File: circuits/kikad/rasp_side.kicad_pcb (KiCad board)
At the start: 2 copper layers, 99.7 x 99.7 mm, 84 parts, among them J1 RJ45, J10 RJ45, J2 RJ45, J3 RJ45, J4 RJ45, J5 RJ45, J6 RJ45, J7 RJ45, J8 RJ45, J9 RJ45

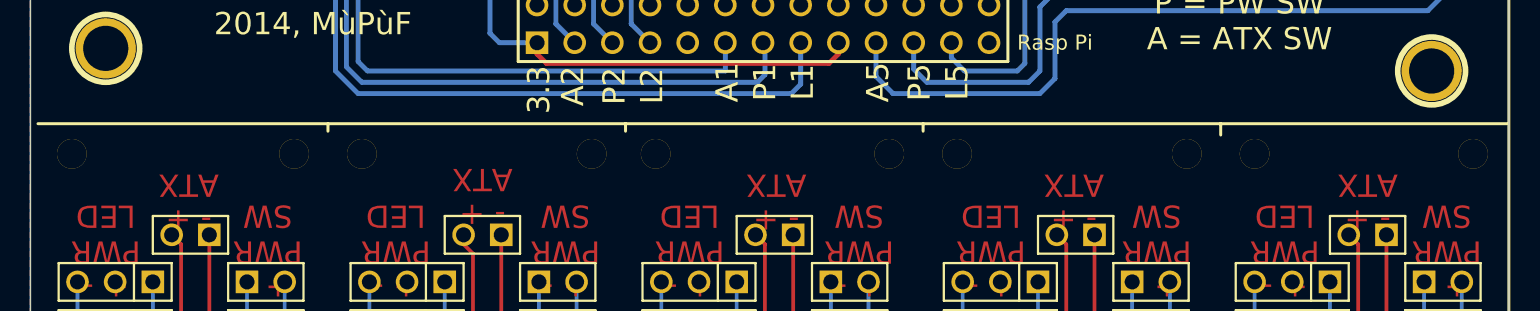
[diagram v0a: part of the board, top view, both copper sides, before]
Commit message: kicad: style fixes
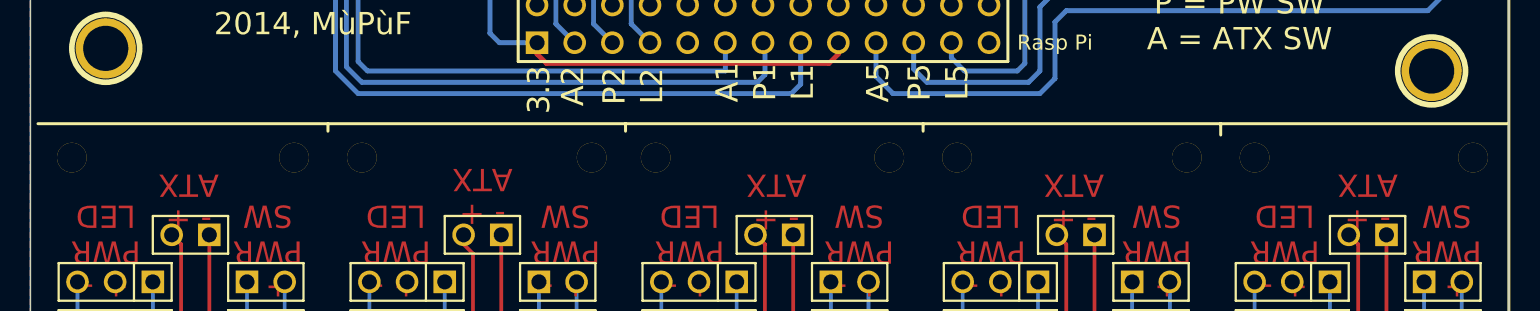
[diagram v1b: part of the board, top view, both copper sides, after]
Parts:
- moved ? 0.25 mm to (13.0, 81.8)
- moved ? 0.25 mm to (27.9, 81.8)
- moved ? 0.25 mm to (32.5, 81.8)
- moved ? 0.25 mm to (48.0, 81.8)
- moved ? 0.25 mm to (52.3, 81.8)
- moved ? 0.25 mm to (68.1, 81.8)
- moved ? 0.25 mm to (72.6, 81.8)
- moved ? 0.25 mm to (88.1, 81.8)
- moved ? 0.25 mm to (92.7, 81.8)
- moved ? 0.25 mm to (107.4, 81.8)
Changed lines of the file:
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@@
     (area 10.059999 5.448299 109.955001 114.312701)
     (thickness 1.6)
-    (drawings 74)
+    (drawings 67)
     (tracks 638)
     (zones 0)
@@
   )
   (module small_hole (layer F.Cu)
-    (at 12.954 81.534)
+    (at 12.954 81.788)
     (descr "module 1 pin (ou trou mecanique de percage)")
     (tags DEV)
@@
   )
   (module small_hole (layer F.Cu)
-    (at 27.94 81.534)
+    (at 27.94 81.788)
     (descr "module 1 pin (ou trou mecanique de percage)")
     (tags DEV)
@@
   )
   (module small_hole (layer F.Cu)
-    (at 32.512 81.534)
+    (at 32.512 81.788)
     (descr "module 1 pin (ou trou mecanique de percage)")
     (tags DEV)
@@
   )
   (module small_hole (layer F.Cu)
-    (at 48.006 81.534)
+    (at 48.006 81.788)
     (descr "module 1 pin (ou trou mecanique de percage)")
     (tags DEV)
@@
   )
   (module small_hole (layer F.Cu)
-    (at 52.324 81.534)
+    (at 52.324 81.788)
     (descr "module 1 pin (ou trou mecanique de percage)")
     (tags DEV)
@@
   )
   (module small_hole (layer F.Cu)
-    (at 68.072 81.534)
+    (at 68.072 81.788)
     (descr "module 1 pin (ou trou mecanique de percage)")
     (tags DEV)
@@
   )
   (module small_hole (layer F.Cu)
-    (at 72.644 81.534)
+    (at 72.644 81.788)
     (descr "module 1 pin (ou trou mecanique de percage)")
     (tags DEV)
@@
   )
   (module small_hole (layer F.Cu)
-    (at 88.138 81.534)
+    (at 88.138 81.788)
     (descr "module 1 pin (ou trou mecanique de percage)")
     (tags DEV)
@@
   )
   (module small_hole (layer F.Cu)
-    (at 92.71 81.534)
+    (at 92.71 81.788)
     (descr "module 1 pin (ou trou mecanique de percage)")
     (tags DEV)
@@
   )
   (module small_hole (layer F.Cu)
-    (at 107.442 81.534)
+    (at 107.442 81.788)
     (descr "module 1 pin (ou trou mecanique de percage)")
     (tags DEV)
@@
     )
   )
+  (gr_text "MùPùF, 2014" (at 20.828 84.074 180) (layer B.SilkS)
+    (effects (font (size 1.5 1.5) (thickness 0.3)) (justify mirror))
+  )
   (gr_line (start 90.424 80.264) (end 90.424 79.502) (angle 90) (layer F.SilkS) (width 0.2))
   (gr_line (start 50.292 80.01) (end 50.292 79.502) (angle 90) (layer F.SilkS) (width 0.2))
@@
   )
   (gr_line (start 30.226 80.264) (end 30.226 109.982) (angle 90) (layer F.Paste) (width 0.2))
-  (gr_text "MùPùF, 2014" (at 21.082 83.82 180) (layer B.SilkS)
-    (effects (font (size 1.5 1.5) (thickness 0.3)) (justify mirror))
-  )
-  (gr_text "MùPùF, 2014" (at 21.082 83.82 180) (layer B.SilkS)
-    (effects (font (size 1.5 1.5) (thickness 0.3)) (justify mirror))
-  )
-  (gr_text "MùPùF, 2014" (at 21.082 83.82 180) (layer B.SilkS)
-    (effects (font (size 1.5 1.5) (thickness 0.3)) (justify mirror))
-  )
-  (gr_text "MùPùF, 2014" (at 21.082 83.82 180) (layer B.SilkS)
-    (effects (font (size 1.5 1.5) (thickness 0.3)) (justify mirror))
-  )
   (gr_line (start 30.226 109.728) (end 30.226 80.01) (angle 90) (layer B.SilkS) (width 0.2))
   (gr_line (start 30.226 80.01) (end 30.226 108.458) (angle 90) (layer B.SilkS) (width 0.2))
@@
   (gr_line (start 30.226 80.01) (end 30.226 108.458) (angle 90) (layer B.SilkS) (width 0.2))
   (gr_line (start 30.226 109.728) (end 30.226 80.01) (angle 90) (layer B.SilkS) (width 0.2))
-  (gr_text "MùPùF, 2014" (at 100.076 83.566 180) (layer B.SilkS)
+  (gr_text "MùPùF, 2014" (at 100.076 84.074 180) (layer B.SilkS)
     (effects (font (size 1.5 1.5) (thickness 0.3)) (justify mirror))
   )
-  (gr_text "MùPùF, 2014" (at 80.518 83.566 180) (layer B.SilkS)
+  (gr_text "MùPùF, 2014" (at 80.264 83.82 180) (layer B.SilkS)
     (effects (font (size 1.5 1.5) (thickness 0.3)) (justify mirror))
   )
@@
     (effects (font (size 1.5 1.5) (thickness 0.3)) (justify mirror))
   )
-  (gr_text "MùPùF, 2014" (at 40.64 83.82 180) (layer B.SilkS)
-    (effects (font (size 1.5 1.5) (thickness 0.3)) (justify mirror))
-  )
-  (gr_text "MùPùF, 2014" (at 21.082 83.82 180) (layer B.SilkS)
-    (effects (font (size 1.5 1.5) (thickness 0.3)) (justify mirror))
-  )
-  (gr_text "MùPùF, 2014" (at 21.082 83.82 180) (layer B.SilkS)
-    (effects (font (size 1.5 1.5) (thickness 0.3)) (justify mirror))
-  )
-  (gr_text "MùPùF, 2014" (at 21.082 83.82 180) (layer B.SilkS)
-    (effects (font (size 1.5 1.5) (thickness 0.3)) (justify mirror))
-  )
-  (gr_text "MùPùF, 2014" (at 21.082 83.82 180) (layer B.SilkS)
+  (gr_text "MùPùF, 2014" (at 40.132 84.074 180) (layer B.SilkS)
     (effects (font (size 1.5 1.5) (thickness 0.3)) (justify mirror))
   )
